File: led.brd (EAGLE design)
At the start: 58 x 58 mm, 47 parts, among them U1 TPS92513, U2 TPS92513

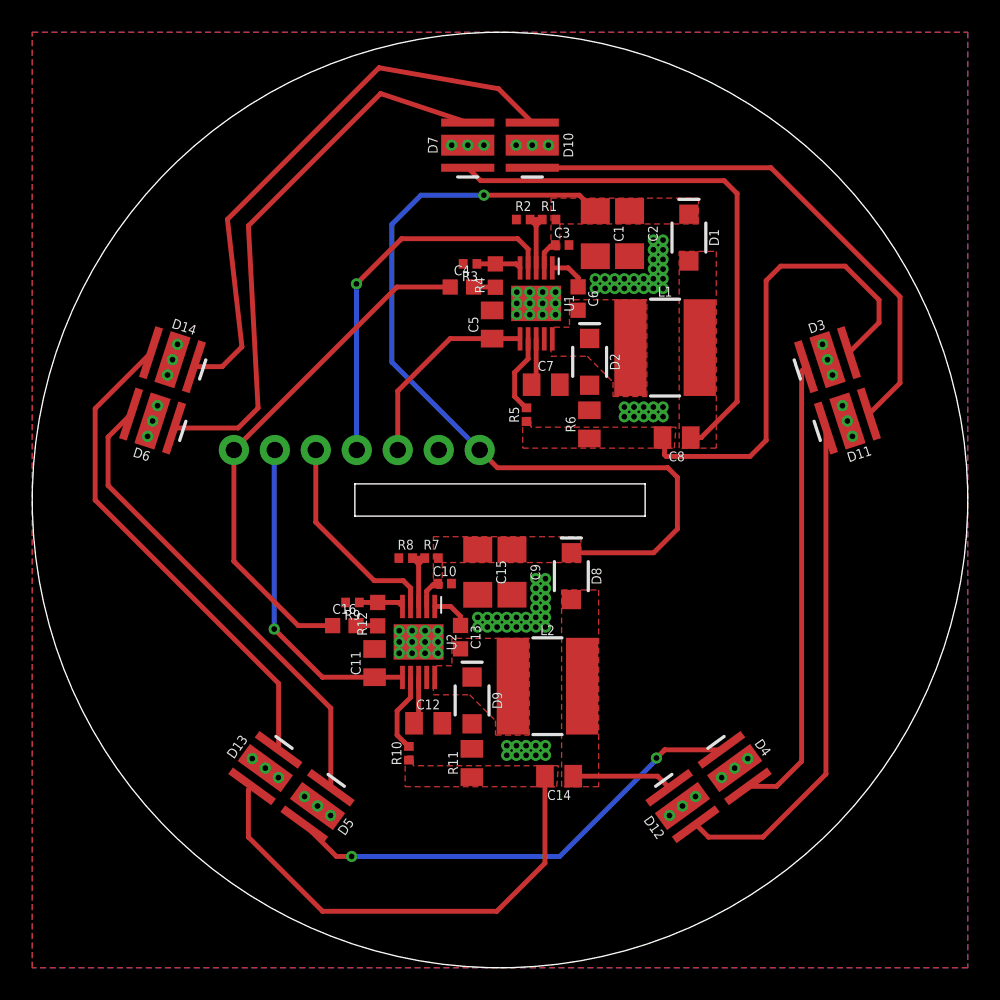
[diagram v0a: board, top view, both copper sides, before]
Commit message: save
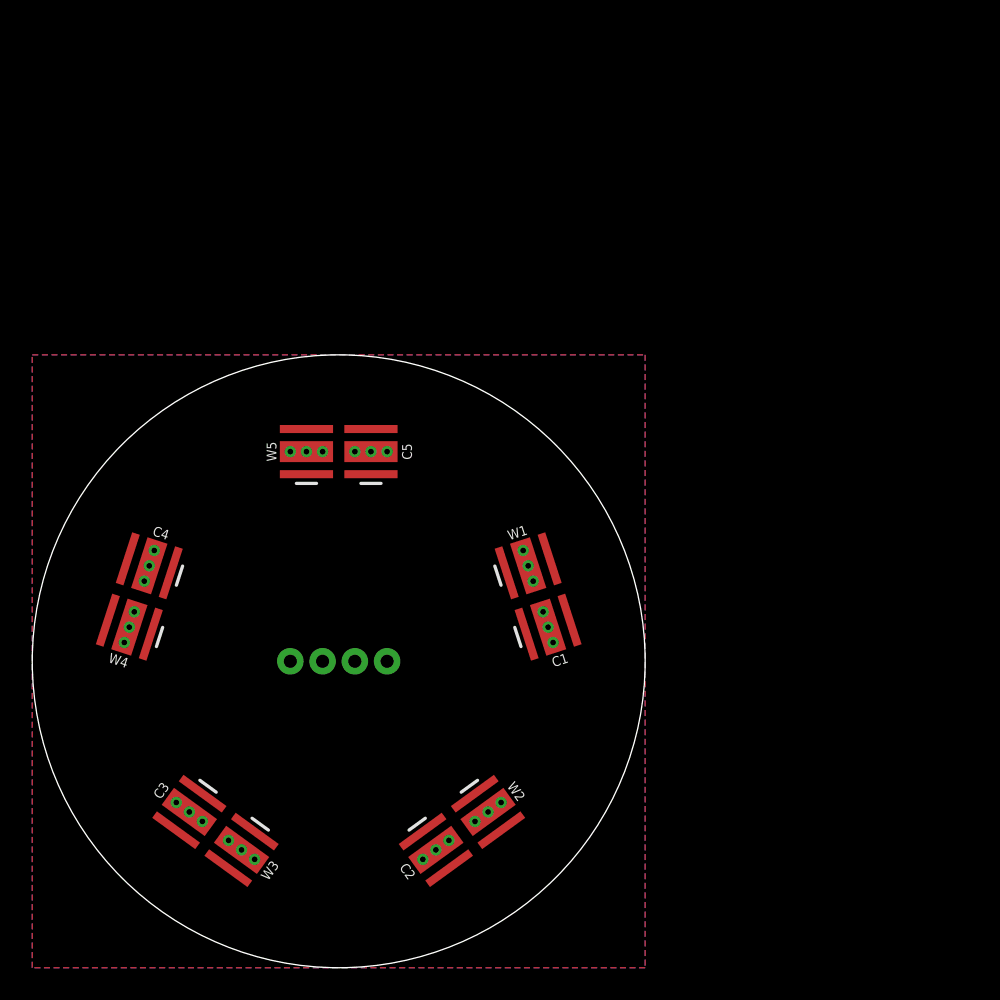
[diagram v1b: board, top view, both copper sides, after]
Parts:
- removed C10: 10000pF, derek:0402
- removed C11: 0.01μF, derek:0805
- removed C12, C7: 0.1µF, derek:0805
- removed C13, C6: 0.1µF, derek:0603
- removed C14, C8: 1µF, derek:0805
- removed C15, C9: 1µF, derek:1206
- removed C16: 470pF, derek:0603
- removed D1, D2, D8, D9: PMEG6010CEH,115, derek:SOD-123F
- removed D10, D11, D12, D13, D14, D3, D4, D5, D6, D7: XPGWHT-L1-0000-00BE8, derek:XLAMP-XPG
- removed J45: (no value), derek:1X07_NO_SILK
- removed L1, L2: 33µH, derek:SRN6045
- removed R1, R7: 97.6k, derek:0402
- removed R10, R5: 976, derek:0402
- removed R11, R6: 0.51, derek:0805
- removed R12, R4: 4.02k, derek:0603
- removed R2, R8: 5.49k, derek:0402
- removed R3, R9: 162k, derek:0402
- removed U1, U2: TPS92513, derek:TPS92513
- added C+, C-, W+, W-: TP-1502, derek:TP-1502
- added W1, W2, W3, W4, W5: XPGWHT-L1-0000-00BE8, derek:XLAMP-XPG
- C1, C2: value 1µF -> XPGWHT-L1-0000-00BE8; device derek:1206 -> derek:XLAMP-XPG
- C3: value 10000pF -> XPGWHT-L1-0000-00BE8; device derek:0402 -> derek:XLAMP-XPG
- C4: value 470pF -> XPGWHT-L1-0000-00BE8; device derek:0603 -> derek:XLAMP-XPG
- C5: value 0.01μF -> XPGWHT-L1-0000-00BE8; device derek:0805 -> derek:XLAMP-XPG
- moved C3 42.1 mm to (9.74, 9.66), turned to 234 degrees
- moved C2 40.1 mm to (25.0, 7.31), turned to 306 degrees
- moved C4 26.0 mm to (7.25, 24.9), turned to 162 degrees
- moved C1 24.6 mm to (32.0, 21.1), turned to 18 degrees
- moved C5 10.9 mm to (21.0, 32.0)
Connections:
- removed net 24V: C1.1, C10.1, C15.1, C2.1, C3.1, C9.1, D1.C, D8.C, J45.7, R1.1, R7.1, U1.2, U2.2
- removed net CLK: C16.2, C4.2, J45.1
- removed net IADJ1: C5.1, J45.5, U1.6
- removed net IADJ2: C11.1, J45.2, U2.6
- removed net N$10: C6.2, U1.1
- removed net N$11: R5.2, U1.7
- removed net N$16: C13.1, D9.C, L2.1, U2.10
- removed net N$17: R12.2, R9.1, U2.5
- removed net N$18: C12.1, U2.8
- removed net N$19: C13.2, U2.1
- removed net N$20: R10.2, U2.7
- removed net N$23: C14.1, D12.C, D8.A, L2.2
- removed net N$25: C16.1, R12.1
- removed net N$26: C14.2, D13.A, R10.1, R11.1
- removed net N$27: D10.C, D11.A
- removed net N$34: C4.1, R4.1
- removed net N$5: C6.1, D2.C, L1.1, U1.10
- removed net N$6: C8.2, D3.A, R5.1, R6.1
- removed net N$7: C8.1, D1.A, D7.C, L1.2
- removed net N$8: R3.1, R4.2, U1.5
- removed net N$9: C7.1, U1.8
- removed net PDIM1: J45.4, U1.4
- removed net PDIM2: J45.3, U2.4
- new net N$30: W+.1, W1.A
- new net N$31: W-.1, W5.C
- new net N$4: C-.1, C5.C
- net GND-ISO: now also C1.GND, C1.P$1, C1.P$2, C1.P$3, C2.GND, C2.P$1, C2.P$2, C2.P$3, C3.GND, C3.P$1, C3.P$2, C3.P$3, C4.GND, C4.P$1, C4.P$2, C4.P$3, C5.GND, C5.P$1, C5.P$2, C5.P$3, W1.GND, W1.P$1, W1.P$2, W1.P$3, W2.GND, W2.P$1, W2.P$2, W2.P$3, W3.GND, W3.P$1, W3.P$2, W3.P$3, W4.GND, W4.P$1, W4.P$2, W4.P$3, W5.GND, W5.P$1, W5.P$2, W5.P$3; no longer C1.2, C10.2, C11.2, C12.2, C15.2, C2.2, C3.2, C5.2, C7.2, C9.2, D10.GND, D10.P$1, D10.P$2, D10.P$3, D11.GND, D11.P$1, D11.P$2, D11.P$3, D12.GND, D12.P$1, D12.P$2, D12.P$3, D13.GND, D13.P$1, D13.P$2, D13.P$3, D14.GND, D14.P$1, D14.P$2, D14.P$3, D2.A, D3.GND, D3.P$1, D3.P$2, D3.P$3, D4.GND, D4.P$1, D4.P$2, D4.P$3, D5.GND, D5.P$1, D5.P$2, D5.P$3, D6.GND, D6.P$1, D6.P$2, D6.P$3, D7.GND, D7.P$1, D7.P$2, D7.P$3, D9.A, J45.6, R11.2, R2.2, R3.2, R6.2, R8.2, R9.2, U1.9, U1.GND-ISO, U1.P$1, U1.P$10, U1.P$11, U1.P$12, U1.P$2, U1.P$3, U1.P$4, U1.P$5, U1.P$6, U1.P$7, U1.P$8, U1.P$9, U2.9, U2.GND-ISO, U2.P$1, U2.P$10, U2.P$11, U2.P$12, U2.P$2, U2.P$3, U2.P$4, U2.P$5, U2.P$6, U2.P$7, U2.P$8, U2.P$9
- net N$1: now also C2.C, C3.A; no longer R7.2, R8.1, U2.3
- net N$12: now also W4.C, W5.A; no longer D6.C, D7.A
- net N$13: now also W1.C, W2.A; no longer D3.C, D4.A
- net N$14: now also W2.C, W3.A; no longer D4.C, D5.A
- net N$15: now also W3.C, W4.A; no longer D5.C, D6.A
- net N$2: now also C1.C, C2.A; no longer D11.C, D12.A
- net N$22: now also C3.C, C4.A; no longer D13.C, D14.A
- net N$24: now also C4.C, C5.A; no longer D10.A, D14.C
- net N$3: now also C+.1, C1.A; no longer R1.2, R2.1, U1.3
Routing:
- net 24V: track 57.0 -> 0.00 mm, vias 1 -> 0
- net N$24: track 35.2 -> 0.00 mm
- net N$12: track 34.3 -> 0.00 mm
- net N$27: track 34.2 -> 0.00 mm
- net N$7: track 34.1 -> 0.00 mm
- net CLK: track 32.3 -> 0.00 mm
- net N$2: track 31.5 -> 0.00 mm
- net N$22: track 30.8 -> 0.00 mm
- net N$26: track 30.2 -> 0.00 mm
- net N$6: track 30.1 -> 0.00 mm
- net N$14: track 29.5 -> 0.00 mm, vias 2 -> 0
- net N$15: track 29.5 -> 0.00 mm
- net N$13: track 28.6 -> 0.00 mm
- net PDIM1: track 23.5 -> 0.00 mm, vias 1 -> 0
- net IADJ2: track 20.3 -> 0.00 mm, vias 1 -> 0
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- removed copper zone on layer 1, net 24V
- removed copper zone on layer 1, net N$16
- removed copper zone on layer 1, net N$23
- removed copper zone on layer 1, net N$26
- removed copper zone on layer 1, net N$5
- removed copper zone on layer 1, net N$6
- removed copper zone on layer 1, net N$7
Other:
- board size 58 x 58 mm -> 38 x 38 mm
